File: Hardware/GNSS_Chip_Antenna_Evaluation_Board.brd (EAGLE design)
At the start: 61 x 35.6 mm, 74 parts, among them J1 U.FL, J2 U.FL, J3 U.FL, J4 U.FL, J5 U.FL, J6 U.FL, Y2 PUCK, Y3 CUBE, Y4 CHIP, Y5 MOLDED, Y6 W3062A, Y7 W3011

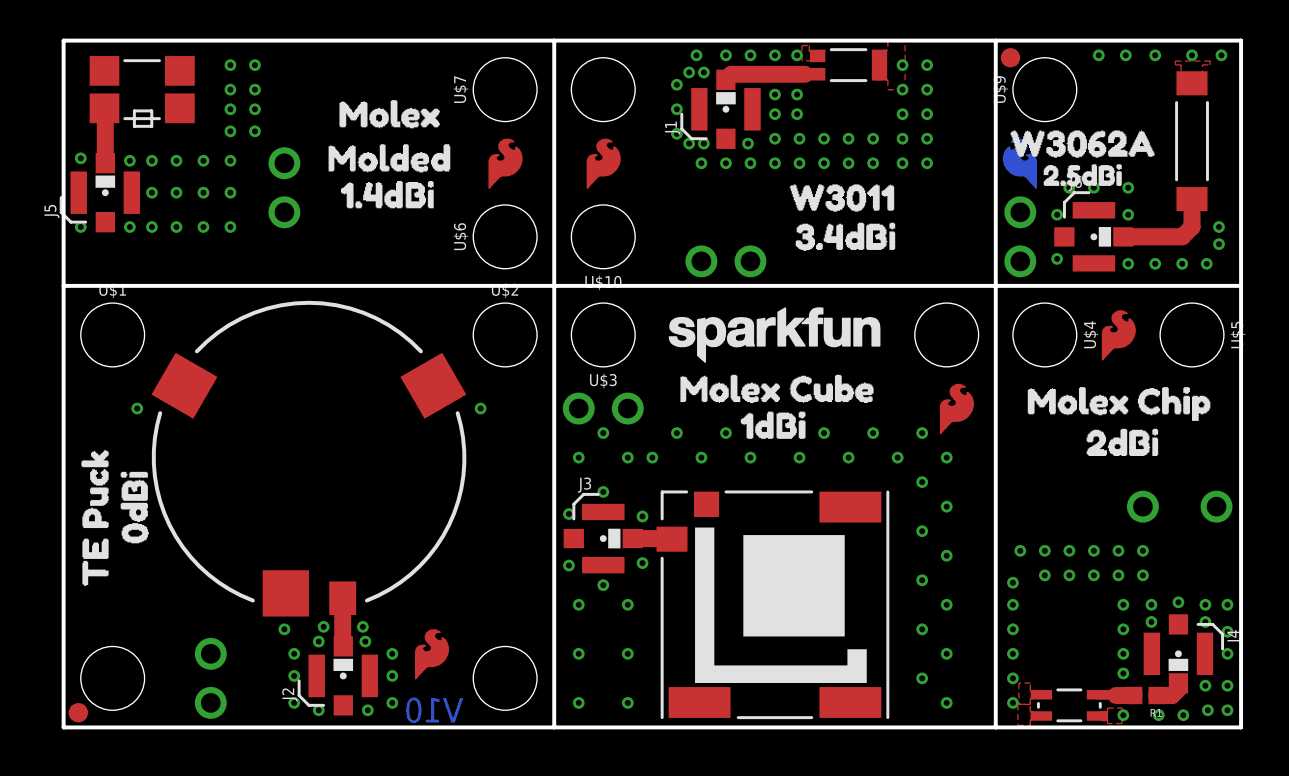
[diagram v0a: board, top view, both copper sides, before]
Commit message: Add schematic title. Bump fiducials. Move version #.
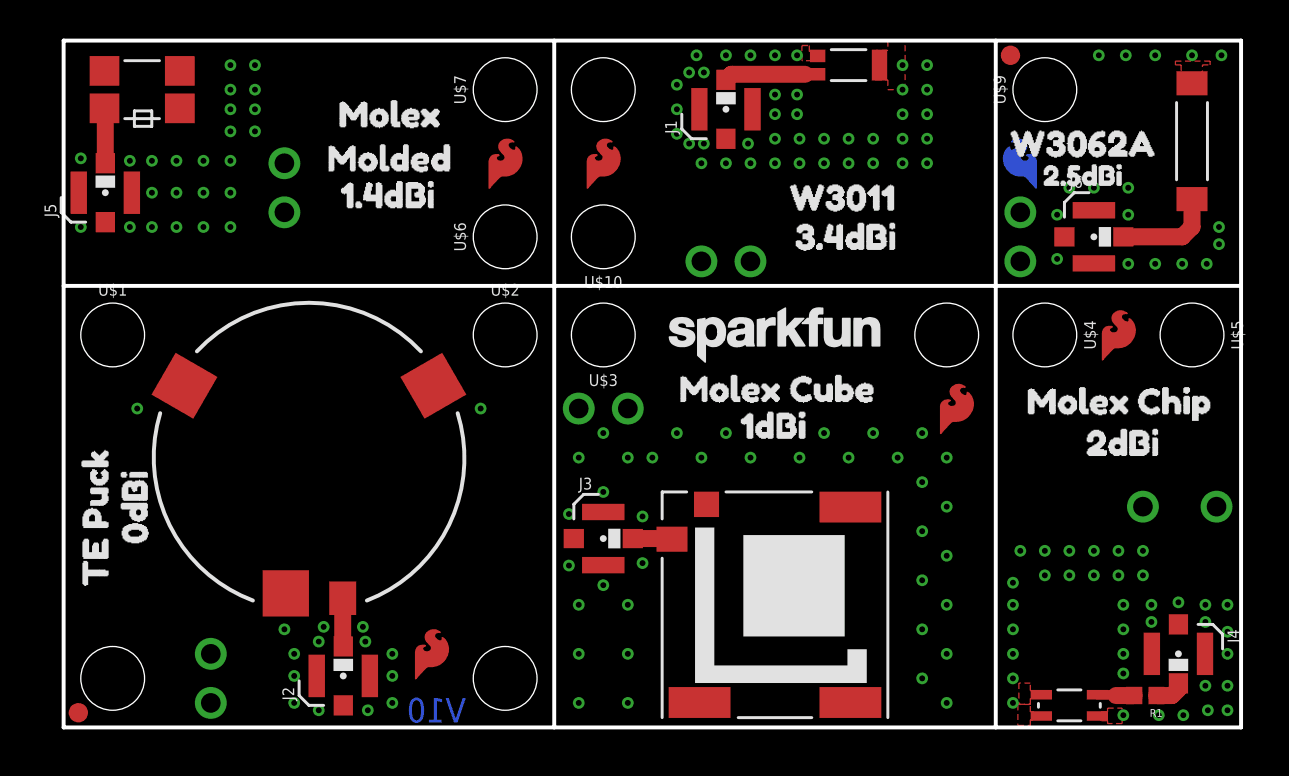
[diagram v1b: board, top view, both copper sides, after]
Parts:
- moved FRAME1 3.59 mm to (3.81, -12.7)
- moved JP8 0.13 mm to (49.0, 34.8)
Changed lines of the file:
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@@
 <layer number="44" name="Drills" color="7" fill="1" visible="no" active="yes"/>
 <layer number="45" name="Holes" color="7" fill="1" visible="yes" active="yes"/>
-<layer number="46" name="Milling" color="3" fill="1" visible="yes" active="yes"/>
-<layer number="47" name="Measures" color="7" fill="1" visible="yes" active="yes"/>
+<layer number="46" name="Milling" color="3" fill="1" visible="no" active="yes"/>
+<layer number="47" name="Measures" color="7" fill="1" visible="no" active="yes"/>
 <layer number="48" name="Document" color="7" fill="1" visible="no" active="yes"/>
 <layer number="49" name="ReferenceLC" color="13" fill="1" visible="no" active="yes"/>
@@
 <wire x1="0" y1="0" x2="0" y2="35.56" width="0.2032" layer="20"/>
 <text x="0" y="-0.0635" size="0.0254" layer="214" font="vector">D:/SmartProjects/Snc/a4_bn_logo2.bmp</text>
-<text x="20.701" y="0.254" size="1.27" layer="16" font="vector" ratio="20" rot="MR0">V10</text>
+<text x="19.304" y="0.889" size="1.27" layer="16" font="vector" ratio="20" rot="MR0" align="center">V10</text>
 <wire x1="25.4" y1="35.56" x2="25.4" y2="0" width="0.2032" layer="20"/>
 <text x="67.31" y="39.37" size="1.27" layer="51">0.8mm Board Thickness</text>
@@
 <element name="JP5" library="SparkFun" package="STAND-OFF" value="STAND-OFF" x="45.72" y="20.32" smashed="yes" rot="R180"/>
 <element name="JP6" library="SparkFun" package="STAND-OFF" value="STAND-OFF" x="27.94" y="33.02" smashed="yes" rot="R180"/>
-<element name="JP8" library="SparkFun" package="FIDUCIAL-1X2" value="FIDUCIAL1X2" x="49.022" y="34.671" smashed="yes"/>
+<element name="JP8" library="SparkFun" package="FIDUCIAL-1X2" value="FIDUCIAL1X2" x="49.022" y="34.798" smashed="yes"/>
 <element name="JP9" library="SparkFun" package="FIDUCIAL-1X2" value="FIDUCIAL1X2" x="0.762" y="0.762" smashed="yes"/>
 <element name="U$16" library="SparkFun-Aesthetics" package="OSHW-LOGO-S" value="OSHW-LOGOS" x="36.83" y="2.54" smashed="yes" rot="MR0"/>
-<element name="FRAME1" library="SparkFun-Aesthetics" package="CREATIVE_COMMONS" value="FRAME-LETTER" x="1.27" y="-15.24" smashed="yes">
-<attribute name="DESIGNER" value="" x="1.27" y="-15.24" size="1.778" layer="27" font="vector" ratio="15" display="off"/>
-<attribute name="REV" value="" x="1.27" y="-15.24" size="1.778" layer="27" font="vector" ratio="15" display="off"/>
-</element>
 <element name="J1" library="SparkFun-Connectors" package="U.FL" value="U.FL" x="34.29" y="32.004" smashed="yes" rot="R90">
 <attribute name="NAME" x="31.75" y="30.734" size="0.6096" layer="25" font="vector" ratio="20" rot="R90"/>
@@
 <element name="U$35" library="buzzard_labels (1)" package="W3062A3" value="" x="53.848" y="35.814" smashed="yes" rot="MR270"/>
 <element name="U$37" library="SparkFun-Aesthetics" package="SFE_LOGO_NAME_FLAME_.1" value="" x="12.827" y="9.652" smashed="yes" rot="MR0"/>
+<element name="FRAME1" library="SparkFun-Aesthetics" package="CREATIVE_COMMONS" value="FRAME-LETTER" x="3.81" y="-12.7" smashed="yes">
+<attribute name="DESIGNER" value="" x="3.81" y="-12.7" size="1.778" layer="27" font="vector" ratio="15" display="off"/>
+<attribute name="REV" value="" x="3.81" y="-12.7" size="1.778" layer="27" font="vector" ratio="15" display="off"/>
+</element>
 </elements>
 <signals>
@@
 <contactref element="Y7" pad="1"/>
 <wire x1="38.7934" y1="33.815" x2="39.04" y2="33.815" width="0.1524" layer="1"/>
-<wire x1="38.387" y1="33.815" x2="39.04" y2="33.815" width="0.2032" layer="1"/>
 <wire x1="34.29" y1="33.529" x2="34.576" y2="33.815" width="0.878840625" layer="1"/>
-<wire x1="34.576" y1="33.815" x2="38.387" y2="33.815" width="0.878840625" layer="1"/>
+<wire x1="38.387" y1="33.815" x2="34.576" y2="33.815" width="0.878840625" layer="1"/>
+<wire x1="39.04" y1="33.815" x2="38.387" y2="33.815" width="0.1524" layer="1"/>
 </signal>
 <signal name="FEED3">
@@
 <contactref element="J3" pad="FEED"/>
 <contactref element="Y3" pad="FEED"/>
-<wire x1="31.36158125" y1="9.779" x2="31.39058125" y2="9.75" width="0.878840625" layer="1"/>
 <wire x1="29.465" y1="9.779" x2="31.36158125" y2="9.779" width="0.878840625" layer="1"/>
 <wire x1="31.5" y1="9.75" x2="31.471" y2="9.779" width="0.2032" layer="1"/>
@@
 <contactref element="J5" pad="FEED"/>
 <wire x1="2.159" y1="29.211003125" x2="2.159" y2="32.004996875" width="0.878840625" layer="1"/>
-<wire x1="2.159" y1="32.004996875" x2="2.114" y2="32.049996875" width="0.878840625" layer="1"/>
 <wire x1="2.114" y1="32.05" x2="2.159" y2="32.005" width="0.2032" layer="1"/>
 <wire x1="2.159" y1="32.005" x2="2.159" y2="32.004996875" width="0.2032" layer="1"/>
